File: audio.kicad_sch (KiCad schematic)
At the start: 60 parts, among them IC1 TAC5212IRGER, J13 Headphones 3.5mm, J18 GUITAR INPUT, J19 LINE OUT LEFT, J20 LINE OUT RIGHT, J22 BALANCED LINE INPUT, SW11 EM-02-Q, U14 OPA1656ID

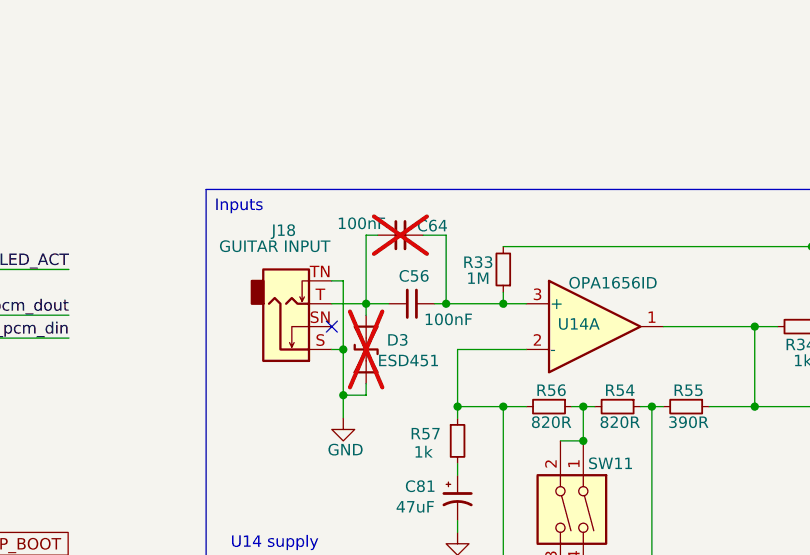
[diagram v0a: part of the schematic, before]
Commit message: opamp incl power routed
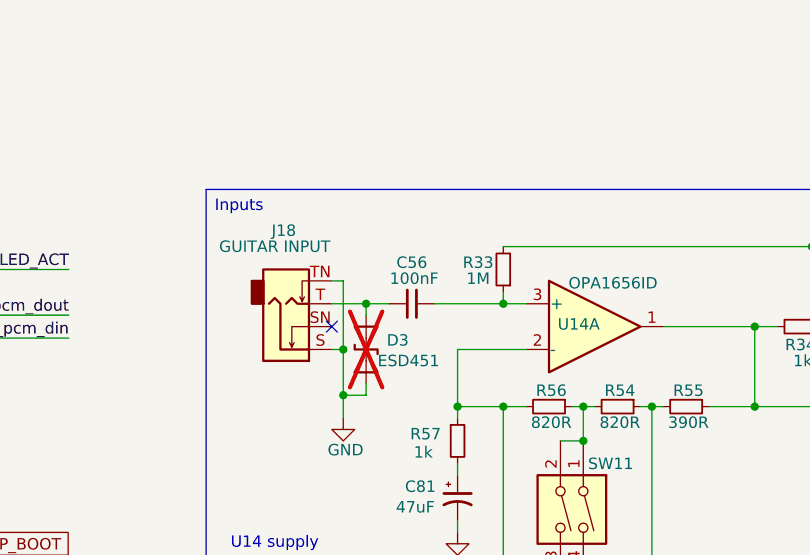
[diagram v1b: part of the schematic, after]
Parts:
- removed C64: 100nF, Capacitor_SMD:C_1206_3216Metric_Pad1.33x1.80mm_HandSolder, symbol Device:C_Small
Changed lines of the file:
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@@
 	)
 	(junction
-		(at 180.34 46.99)
-		(diameter 0)
-		(color 0 0 0 0)
-	)
-	(junction
 		(at 91.44 184.15)
 		(diameter 0)
@@
 	(wire
 		(pts
-			(xy 180.34 39.37) (xy 180.34 46.99)
-		)
-		(stroke
-			(width 0)
-			(type default)
-		)
-	)
-	(wire
-		(pts
 			(xy 74.93 175.26) (xy 74.93 173.99)
 		)
@@
 	(wire
 		(pts
-			(xy 177.8 39.37) (xy 180.34 39.37)
-		)
-		(stroke
-			(width 0)
-			(type default)
-		)
-	)
-	(wire
-		(pts
 			(xy 179.07 46.99) (xy 189.23 46.99)
 		)
@@
 	(wire
 		(pts
-			(xy 172.72 39.37) (xy 171.45 39.37)
-		)
-		(stroke
-			(width 0)
-			(type default)
-		)
-	)
-	(wire
-		(pts
 			(xy 190.5 153.67) (xy 194.31 153.67)
 		)
@@
 	(wire
 		(pts
-			(xy 171.45 39.37) (xy 171.45 46.99)
-		)
-		(stroke
-			(width 0)
-			(type default)
-		)
-	)
-	(wire
-		(pts
 			(xy 168.91 57.15) (xy 171.45 57.15)
 		)
@@
 	)
 	(symbol
-		(lib_id "Device:C_Small")
-		(at 175.26 39.37 90)
-		(unit 1)
-		(body_style 1)
-		(exclude_from_sim no)
-		(in_bom yes)
-		(on_board yes)
-		(in_pos_files yes)
-		(dnp yes)
-		(property "Reference" "C64"
-			(at 178.816 38.354 90)
-			(show_name no)
-			(do_not_autoplace no)
-			(effects
-				(font
-					(size 1.27 1.27)
-				)
-			)
-		)
-		(property "Value" "100nF"
-			(at 170.942 38.1 90)
-			(show_name no)
-			(do_not_autoplace no)
-			(effects
-				(font
-					(size 1.27 1.27)
-				)
-			)
-		)
-		(property "Footprint" "Capacitor_SMD:C_1206_3216Metric_Pad1.33x1.80mm_HandSolder"
-			(at 175.26 39.37 0)
-			(hide yes)
-			(show_name no)
-			(do_not_autoplace no)
-			(effects
-				(font
-					(size 1.27 1.27)
-				)
-			)
-		)
-		(property "Datasheet" ""
-			(at 175.26 39.37 0)
-			(hide yes)
-			(show_name no)
-			(do_not_autoplace no)
-			(effects
-				(font
-					(size 1.27 1.27)
-				)
-			)
-		)
-		(property "Description" "C0G alternative"
-			(at 175.26 39.37 0)
-			(hide yes)
-			(show_name no)
-			(do_not_autoplace no)
-			(effects
-				(font
-					(size 1.27 1.27)
-				)
-			)
-		)
-		(pin "2"
-		)
-		(pin "1"
-		)
-		(instances
-			(project "pedalboard-hw"
-				(path "/df521c2a-9827-4355-b809-366f4b88d5d7/6bd0afd4-cd8b-4c1d-a236-891eed0b2d91"
-					(reference "C64")
-					(unit 1)
-				)
-			)
-		)
-	)
-	(symbol
 		(lib_id "Connector_Audio:AudioJack3_SwitchTR")
 		(at 252.73 121.92 180)
@@
 		(dnp no)
 		(property "Reference" "C56"
-			(at 176.784 43.942 90)
+			(at 176.53 42.418 90)
 			(show_name no)
 			(do_not_autoplace no)
@@
 		)
 		(property "Value" "100nF"
-			(at 180.594 48.768 90)
+			(at 176.784 44.196 90)
 			(show_name no)
 			(do_not_autoplace no)
